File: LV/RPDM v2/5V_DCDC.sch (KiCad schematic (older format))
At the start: 4 parts

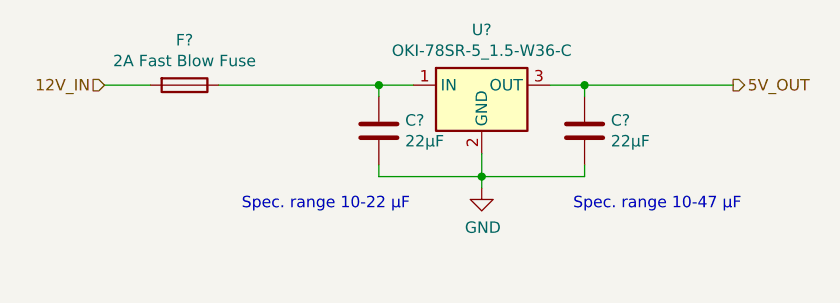
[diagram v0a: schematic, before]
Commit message: rpdm
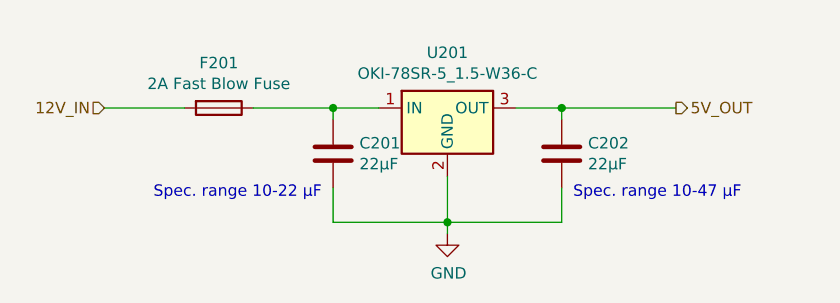
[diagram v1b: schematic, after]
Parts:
- gave numbers to parts that had none: 4
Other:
- moved on the sheet: C201, C202, F201, U201
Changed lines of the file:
@@
 $Descr A4 11693 8268
 encoding utf-8
-Sheet 4 30
+Sheet 2 30
 Title ""
 Date "2021-06-28"
@@
 $EndDescr
 $Comp
-L RPDM-v2-rescue:OKI-78SR-5_1.5-W36-C-Converter_DCDC-RPDM-v1-rescue U?
+L RPDM-v2-rescue:OKI-78SR-5_1.5-W36-C-Converter_DCDC-RPDM-v1-rescue U201
 U 1 1 61024FA3
-P 5650 3400
-AR Path="/5E553FD7/61024FA3" Ref="U?"  Part="1"
+P 5500 3500
+AR Path="/5E553FD7/61024FA3" Ref="U201"  Part="1"
 AR Path="/5E553FD7/6101A8C0/61024FA3" Ref="U?"  Part="1"
 AR Path="/5E553FD7/61027E0C/61024FA3" Ref="U?"  Part="1"
-F 0 "U?" H 5650 3642 50  0000 C CNN
-F 1 "OKI-78SR-5_1.5-W36-C" H 5650 3551 50  0000 C CNN
-F 2 "Converter_DCDC:Converter_DCDC_muRata_OKI-78SR_Vertical" H 5700 3150 50  0001 L CIN
-F 3 "https://power.murata.com/data/power/oki-78sr.pdf" H 5650 3400 50  0001 C CNN
-	1    5650 3400
+F 0 "U201" H 5500 3742 50  0000 C CNN
+F 1 "OKI-78SR-5_1.5-W36-C" H 5500 3651 50  0000 C CNN
+F 2 "Converter_DCDC:Converter_DCDC_muRata_OKI-78SR_Vertical" H 5550 3250 50  0001 L CIN
+F 3 "https://power.murata.com/data/power/oki-78sr.pdf" H 5500 3500 50  0001 C CNN
+	1    5500 3500
 	1    0    0    -1
 $EndComp
-Text HLabel 4000 3400 0    50   Input ~ 0
+Text HLabel 4000 3500 0    50   Input ~ 0
 12V_IN
 $Comp
-L Device:C C?
+L Device:C C201
 U 1 1 61024FAA
-P 5200 3600
-AR Path="/5E553FD7/61024FAA" Ref="C?"  Part="1"
+P 5000 3700
+AR Path="/5E553FD7/61024FAA" Ref="C201"  Part="1"
 AR Path="/5E553FD7/6101A8C0/61024FAA" Ref="C?"  Part="1"
 AR Path="/5E553FD7/61027E0C/61024FAA" Ref="C?"  Part="1"
-F 0 "C?" H 5315 3646 50  0000 L CNN
-F 1 "22µF" H 5315 3555 50  0000 L CNN
-F 2 "" H 5238 3450 50  0001 C CNN
-F 3 "~" H 5200 3600 50  0001 C CNN
-	1    5200 3600
+F 0 "C201" H 5115 3746 50  0000 L CNN
+F 1 "22µF" H 5115 3655 50  0000 L CNN
+F 2 "" H 5038 3550 50  0001 C CNN
+F 3 "~" H 5000 3700 50  0001 C CNN
+	1    5000 3700
 	1    0    0    -1
 $EndComp
 $Comp
-L power:GND #PWR?
+L power:GND #PWR0201
 U 1 1 61024FB6
-P 5650 3850
-AR Path="/5E553FD7/61024FB6" Ref="#PWR?"  Part="1"
+P 5500 4050
+AR Path="/5E553FD7/61024FB6" Ref="#PWR0201"  Part="1"
 AR Path="/5E553FD7/6101A8C0/61024FB6" Ref="#PWR?"  Part="1"
 AR Path="/5E553FD7/61027E0C/61024FB6" Ref="#PWR?"  Part="1"
-F 0 "#PWR?" H 5650 3600 50  0001 C CNN
-F 1 "GND" H 5655 3677 50  0000 C CNN
-F 2 "" H 5650 3850 50  0001 C CNN
-F 3 "" H 5650 3850 50  0001 C CNN
-	1    5650 3850
+F 0 "#PWR0201" H 5500 3800 50  0001 C CNN
+F 1 "GND" H 5505 3877 50  0000 C CNN
+F 2 "" H 5500 4050 50  0001 C CNN
+F 3 "" H 5500 4050 50  0001 C CNN
+	1    5500 4050
 	1    0    0    -1
 $EndComp
-Text HLabel 6750 3400 2    50   Output ~ 0
+Text HLabel 6500 3500 2    50   Output ~ 0
 5V_OUT
 Wire Wire Line
-	5950 3400 6100 3400
+	5800 3500 6000 3500
 Wire Wire Line
-	6100 3450 6100 3400
-Connection ~ 6100 3400
+	6000 3550 6000 3500
+Connection ~ 6000 3500
 Wire Wire Line
-	5650 3700 5650 3800
+	6000 4000 6000 3850
 Wire Wire Line
-	5650 3800 6100 3800
+	5200 3500 5000 3500
 Wire Wire Line
-	6100 3800 6100 3750
-Wire Wire Line
-	5350 3400 5200 3400
-Wire Wire Line
-	5200 3400 5200 3450
-Wire Wire Line
-	5200 3750 5200 3800
-Wire Wire Line
-	5200 3800 5650 3800
-Connection ~ 5650 3800
-Connection ~ 5200 3400
-Wire Wire Line
-	5650 3800 5650 3850
+	5000 3500 5000 3550
+Connection ~ 5000 3500
 $Comp
-L Device2:Fuse F?
+L Device2:Fuse F201
 U 1 1 60DABEEF
-P 4350 3400
-F 0 "F?" V 4153 3400 50  0000 C CNN
-F 1 "2A Fast Blow Fuse" V 4244 3400 50  0000 C CNN
-F 2 "" V 4280 3400 50  0001 C CNN
-F 3 "~" H 4350 3400 50  0001 C CNN
-	1    4350 3400
+P 4500 3500
+F 0 "F201" V 4303 3500 50  0000 C CNN
+F 1 "2A Fast Blow Fuse" V 4394 3500 50  0000 C CNN
+F 2 "" V 4430 3500 50  0001 C CNN
+F 3 "~" H 4500 3500 50  0001 C CNN
+	1    4500 3500
 	0    1    1    0
 $EndComp
 Wire Wire Line
-	4000 3400 4200 3400
+	4000 3500 4350 3500
 Wire Wire Line
-	4500 3400 5200 3400
+	4650 3500 5000 3500
 Wire Wire Line
-	6100 3400 6750 3400
+	6000 3500 6500 3500
 $Comp
-L Device:C C?
+L Device:C C202
 U 1 1 61BA18F7
-P 6100 3600
-AR Path="/5E553FD7/61BA18F7" Ref="C?"  Part="1"
+P 6000 3700
+AR Path="/5E553FD7/61BA18F7" Ref="C202"  Part="1"
 AR Path="/5E553FD7/6101A8C0/61BA18F7" Ref="C?"  Part="1"
 AR Path="/5E553FD7/61027E0C/61BA18F7" Ref="C?"  Part="1"
-F 0 "C?" H 6215 3646 50  0000 L CNN
-F 1 "22µF" H 6215 3555 50  0000 L CNN
-F 2 "" H 6138 3450 50  0001 C CNN
-F 3 "~" H 6100 3600 50  0001 C CNN
-	1    6100 3600
+F 0 "C202" H 6115 3746 50  0000 L CNN
+F 1 "22µF" H 6115 3655 50  0000 L CNN
+F 2 "" H 6038 3550 50  0001 C CNN
+F 3 "~" H 6000 3700 50  0001 C CNN
+	1    6000 3700
 	1    0    0    -1
 $EndComp
-Text Notes 4600 3950 0    50   ~ 0
+Text Notes 4950 3900 2    50   ~ 0
 Spec. range 10-22 µF
-Text Notes 6050 3950 0    50   ~ 0
+Text Notes 6050 3900 0    50   ~ 0
 Spec. range 10-47 µF
+Wire Wire Line
+	5500 4000 5500 4050
+Wire Wire Line
+	5500 4000 6000 4000
+Wire Wire Line
+	5500 3800 5500 4000
+Connection ~ 5500 4000
+Wire Wire Line
+	5000 3850 5000 4000
+Wire Wire Line
+	5000 4000 5500 4000
 $EndSCHEMATC
